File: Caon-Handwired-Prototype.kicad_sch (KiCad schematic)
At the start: 27 parts, among them SW1 SW_PUSH_MX, SW2 SW_PUSH_MX, SW3 SW_PUSH_MX, SW4 EC11 ENCODER 1, SW5 SW_PUSH_MX, SW6 SW_PUSH_MX, SW7 SW_PUSH_MX, SW8 EC11 ENCODER 1, U1 74HC595, U2 74HC595, U3 SuperMini nRF52840

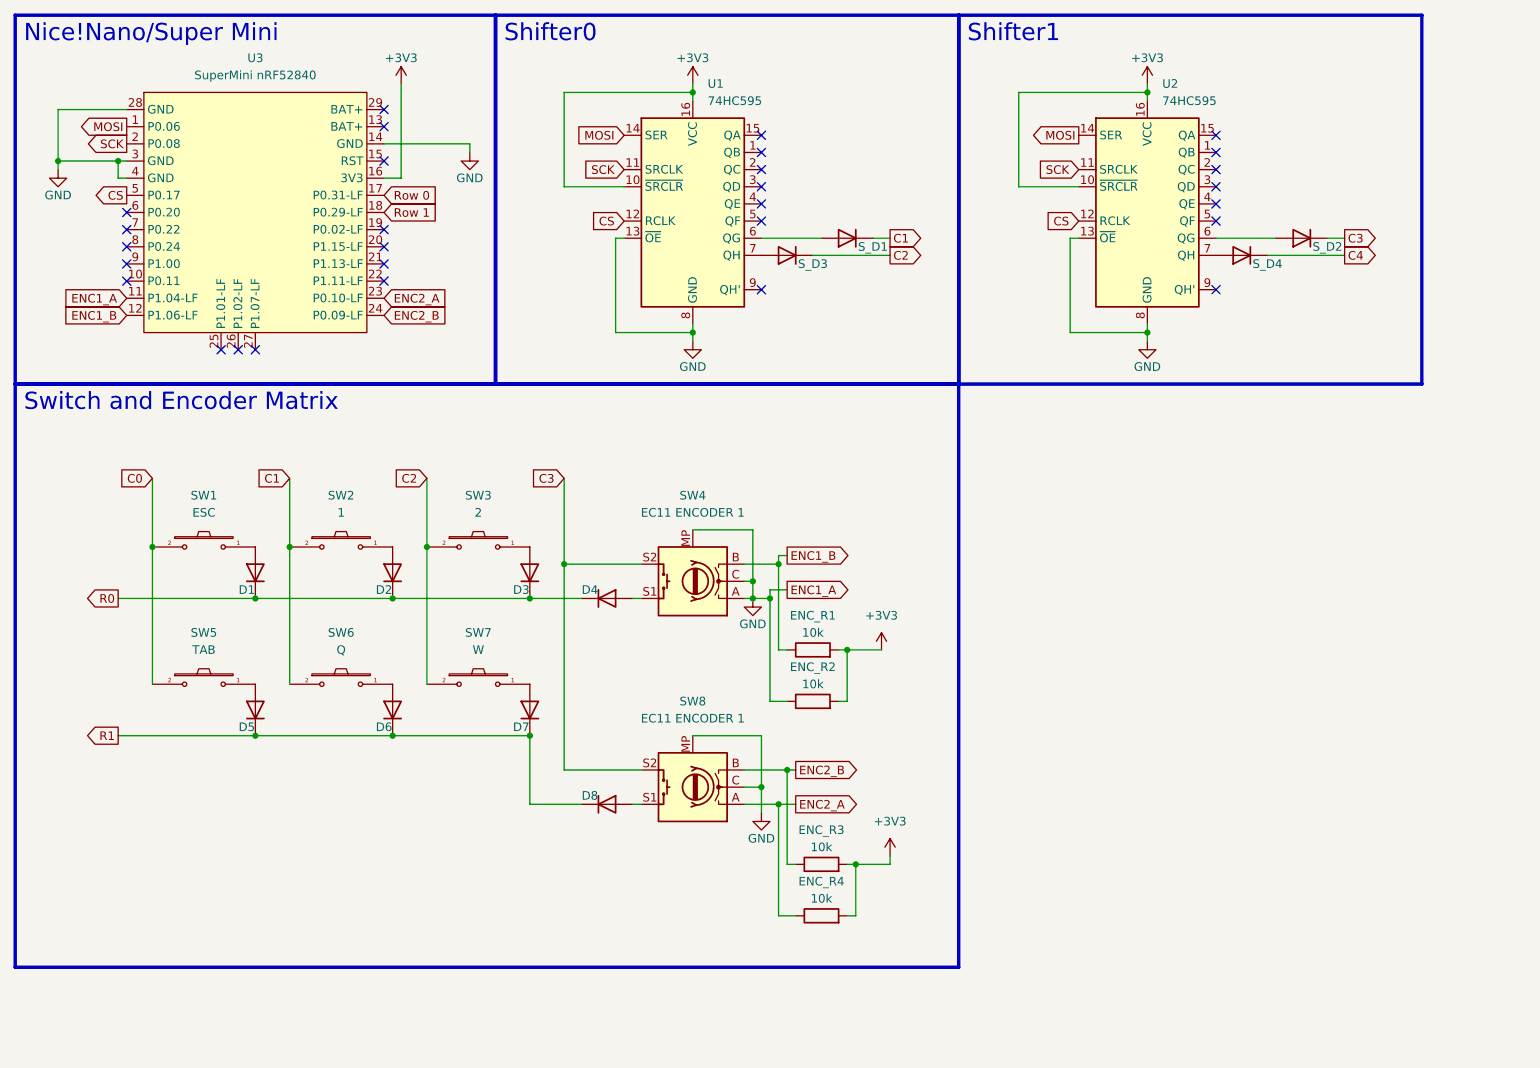
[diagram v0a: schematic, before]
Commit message: Update
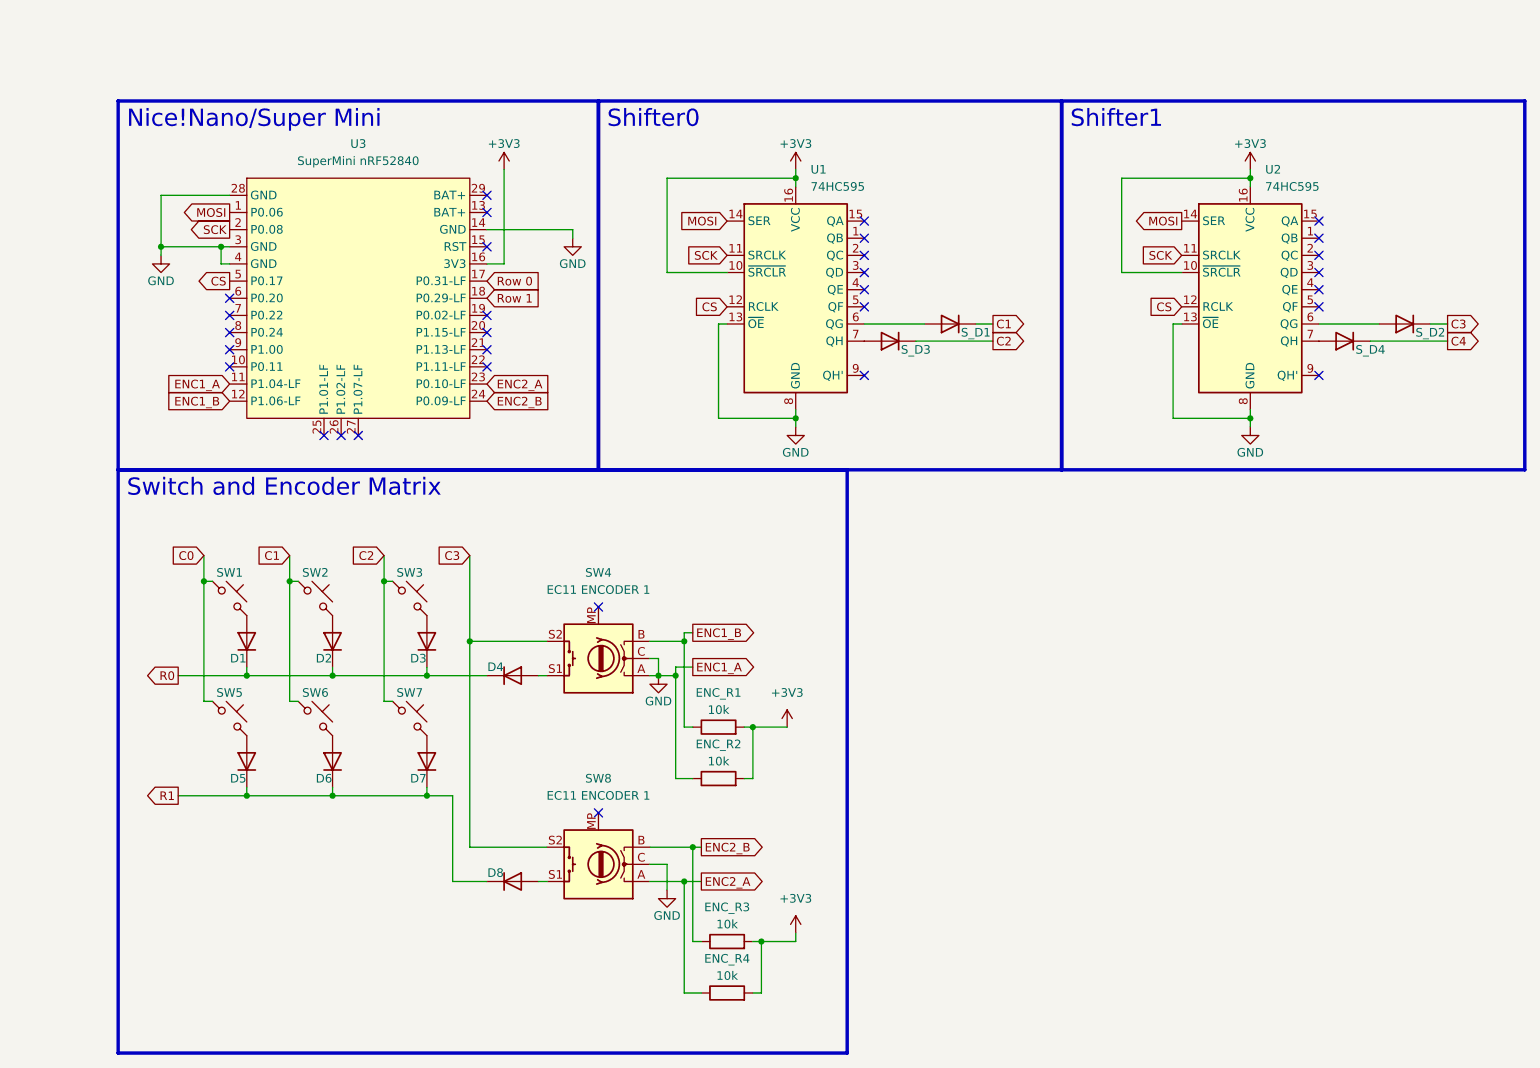
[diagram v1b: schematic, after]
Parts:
- removed SW1, SW2, SW3, SW5, SW6, SW7: SW_PUSH_MX, Caon_Footprint:SW_PUSH_6mm, symbol Caon65:SW_PUSH_MX
- added SW1, SW2, SW3, SW5, SW6, SW7: ~, Caon_Footprint:SW_PUSH_6mm, symbol Switch:SW_Push_45deg
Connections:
- net C0: now also SW1.1, SW5.1
- net C1: now also SW2.1, SW6.1
- net C2: now also SW3.1, SW7.1
- net GND: no longer SW4.MP, SW8.MP
- net at D1.2 (A): now also SW1.2
- net at D3.2 (A): now also SW3.2
- net at D5.2 (A): now also SW5.2
- net at D6.2 (A): now also SW6.2
- net at D2.2 (A): now also SW2.2
- net at D7.2 (A): now also SW7.2
- no-connect marks 29 -> 31
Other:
- moved on the sheet: D1, D4, D8, ENC_R1, ENC_R2, ENC_R3, ENC_R4, SW4, SW8, S_D1, S_D2, S_D3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

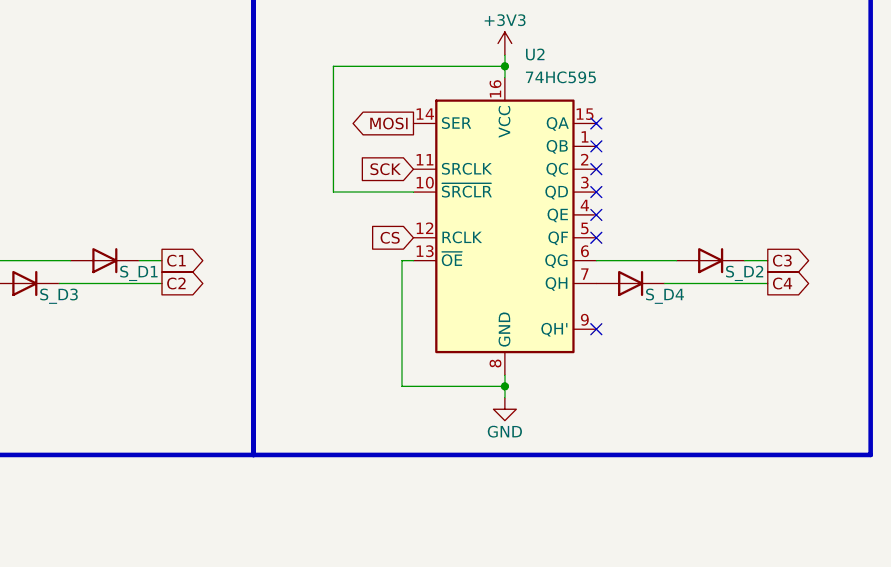
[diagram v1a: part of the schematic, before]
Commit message: Update
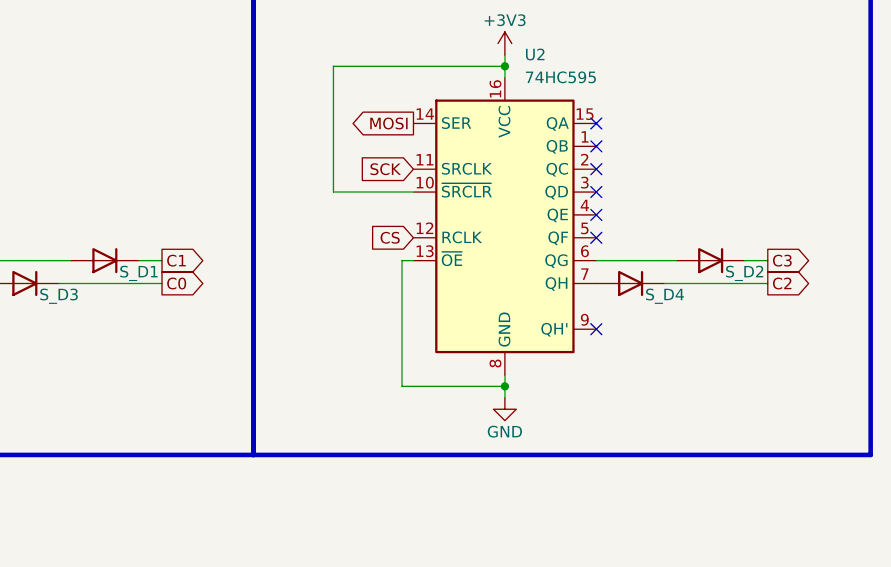
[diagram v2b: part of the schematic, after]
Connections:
- net C4 is gone; now on net C2: S_D4.1 (K)
- net C0: now also S_D3.1 (K)
- net C2: no longer S_D3.1 (K)

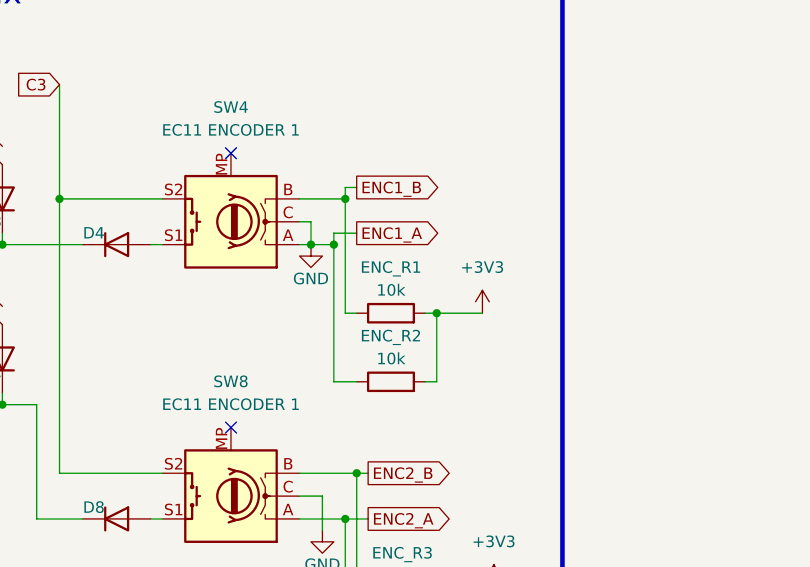
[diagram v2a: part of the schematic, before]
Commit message: Schematic Update
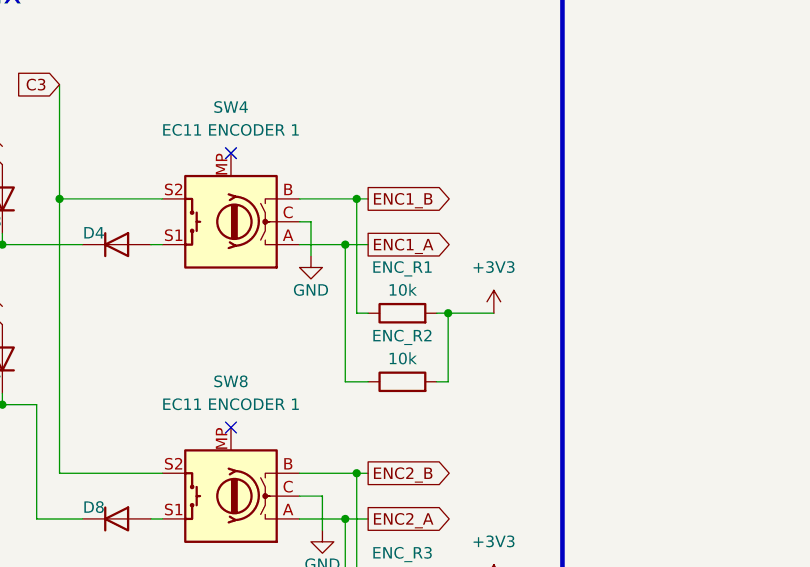
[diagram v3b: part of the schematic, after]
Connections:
- net GND: no longer ENC_R2.1, SW4.A, U3.11 (P1.04-LF)
- new net ENC1_A: ENC_R2.1, SW4.A, U3.11 (P1.04-LF)
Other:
- moved on the sheet: ENC_R1, ENC_R2
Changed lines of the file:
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@@
 	)
 	(junction
-		(at 137.16 125.73)
+		(at 138.43 125.73)
 		(diameter 0)
 		(color 0 0 0 0)
@@
 	)
 	(junction
-		(at 127 113.03)
+		(at 128.27 113.03)
 		(diameter 0)
 		(color 0 0 0 0)
@@
 	)
 	(junction
-		(at 123.19 118.11)
-		(diameter 0)
-		(color 0 0 0 0)
-	)
-	(junction
 		(at 138.43 157.48)
 		(diameter 0)
@@
 	)
 	(junction
-		(at 125.73 118.11)
+		(at 127 118.11)
 		(diameter 0)
 		(color 0 0 0 0)
@@
 	(wire
 		(pts
-			(xy 127 113.03) (xy 121.92 113.03)
-		)
-		(stroke
-			(width 0)
-			(type default)
-		)
-	)
-	(wire
-		(pts
-			(xy 127 125.73) (xy 127 113.03)
+			(xy 128.27 125.73) (xy 128.27 113.03)
 		)
 		(stroke
@@
 	(wire
 		(pts
-			(xy 127 113.03) (xy 127 111.76)
-		)
-		(stroke
-			(width 0)
-			(type default)
-		)
-	)
-	(wire
-		(pts
 			(xy 74.93 118.11) (xy 88.9 118.11)
 		)
@@
 	(wire
 		(pts
-			(xy 125.73 118.11) (xy 125.73 116.84)
-		)
-		(stroke
-			(width 0)
-			(type default)
-		)
-	)
-	(wire
-		(pts
 			(xy 137.16 165.1) (xy 138.43 165.1)
 		)
@@
 	(wire
 		(pts
-			(xy 127 111.76) (xy 128.27 111.76)
+			(xy 128.27 113.03) (xy 129.54 113.03)
 		)
 		(stroke
@@
 	(wire
 		(pts
-			(xy 123.19 118.11) (xy 123.19 115.57)
+			(xy 123.19 115.57) (xy 123.19 119.38)
 		)
 		(stroke
@@
 	(wire
 		(pts
-			(xy 128.27 125.73) (xy 127 125.73)
+			(xy 129.54 125.73) (xy 128.27 125.73)
 		)
 		(stroke
@@
 	(wire
 		(pts
-			(xy 125.73 133.35) (xy 125.73 118.11)
+			(xy 127 133.35) (xy 127 118.11)
 		)
 		(stroke
@@
 	(wire
 		(pts
-			(xy 137.16 133.35) (xy 137.16 125.73)
+			(xy 138.43 133.35) (xy 138.43 125.73)
 		)
 		(stroke
@@
 	(wire
 		(pts
-			(xy 135.89 125.73) (xy 137.16 125.73)
+			(xy 137.16 125.73) (xy 138.43 125.73)
 		)
 		(stroke
@@
 	(wire
 		(pts
-			(xy 125.73 118.11) (xy 123.19 118.11)
+			(xy 74.93 134.62) (xy 74.93 135.89)
 		)
 		(stroke
@@
 	(wire
 		(pts
-			(xy 74.93 134.62) (xy 74.93 135.89)
+			(xy 58.42 54.61) (xy 58.42 57.15)
 		)
 		(stroke
@@
 	(wire
 		(pts
-			(xy 58.42 54.61) (xy 58.42 57.15)
+			(xy 62.23 116.84) (xy 62.23 118.11)
 		)
 		(stroke
@@
 	(wire
 		(pts
-			(xy 62.23 116.84) (xy 62.23 118.11)
+			(xy 128.27 157.48) (xy 128.27 143.51)
 		)
 		(stroke
@@
 	(wire
 		(pts
-			(xy 128.27 157.48) (xy 128.27 143.51)
+			(xy 137.16 133.35) (xy 138.43 133.35)
 		)
 		(stroke
@@
 	(wire
 		(pts
-			(xy 135.89 133.35) (xy 137.16 133.35)
+			(xy 127 118.11) (xy 129.54 118.11)
 		)
 		(stroke
@@
 	(wire
 		(pts
-			(xy 125.73 116.84) (xy 128.27 116.84)
+			(xy 83.82 104.14) (xy 82.55 104.14)
 		)
 		(stroke
@@
 	(wire
 		(pts
-			(xy 83.82 104.14) (xy 82.55 104.14)
+			(xy 100.33 43.18) (xy 100.33 57.15)
 		)
 		(stroke
@@
 	(wire
 		(pts
-			(xy 100.33 43.18) (xy 100.33 57.15)
+			(xy 143.51 81.28) (xy 143.51 80.01)
 		)
 		(stroke
@@
 	(wire
 		(pts
-			(xy 143.51 81.28) (xy 143.51 80.01)
+			(xy 121.92 113.03) (xy 128.27 113.03)
 		)
 		(stroke
@@
 	(wire
 		(pts
-			(xy 128.27 133.35) (xy 125.73 133.35)
+			(xy 129.54 133.35) (xy 127 133.35)
 		)
 		(stroke
@@
 	(wire
 		(pts
-			(xy 123.19 118.11) (xy 121.92 118.11)
+			(xy 121.92 118.11) (xy 127 118.11)
 		)
 		(stroke
@@
 	(wire
 		(pts
-			(xy 137.16 125.73) (xy 142.24 125.73)
+			(xy 138.43 125.73) (xy 143.51 125.73)
 		)
 		(stroke
@@
 	(global_label "ENC1_A"
 		(shape output)
-		(at 128.27 116.84 0)
+		(at 129.54 118.11 0)
 		(fields_autoplaced yes)
 		(effects
@@
 		)
 		(property "Intersheetrefs" "${INTERSHEET_REFS}"
-			(at 138.2704 116.84 0)
+			(at 139.5404 118.11 0)
 			(effects
 				(font
@@
 	(global_label "ENC1_B"
 		(shape output)
-		(at 128.27 111.76 0)
+		(at 129.54 113.03 0)
 		(fields_autoplaced yes)
 		(effects
@@
 		)
 		(property "Intersheetrefs" "${INTERSHEET_REFS}"
-			(at 138.4518 111.76 0)
+			(at 139.7218 113.03 0)
 			(effects
 				(font
@@
 	(symbol
 		(lib_id "power:GND")
-		(at 123.19 118.11 0)
+		(at 123.19 119.38 0)
 		(unit 1)
 		(exclude_from_sim no)
@@
 		(dnp no)
 		(property "Reference" "#PWR08"
-			(at 123.19 124.46 0)
+			(at 123.19 125.73 0)
 			(effects
 				(font
@@
 		)
 		(property "Value" "GND"
-			(at 123.19 121.92 0)
+			(at 123.19 123.19 0)
 			(effects
 				(font
@@
 		)
 		(property "Footprint" ""
-			(at 123.19 118.11 0)
+			(at 123.19 119.38 0)
 			(effects
 				(font
@@
 		)
 		(property "Datasheet" ""
-			(at 123.19 118.11 0)
+			(at 123.19 119.38 0)
 			(effects
 				(font
@@
 		)
 		(property "Description" "Power symbol creates a global label with name \"GND\" , ground"
-			(at 123.19 118.11 0)
+			(at 123.19 119.38 0)
 			(effects
 				(font
@@
 	(symbol
 		(lib_id "Device:R")
-		(at 132.08 125.73 90)
+		(at 133.35 125.73 90)
 		(unit 1)
 		(exclude_from_sim no)
@@
 		(dnp no)
 		(property "Reference" "ENC_R1"
-			(at 132.08 120.65 90)
+			(at 133.35 120.65 90)
 			(effects
 				(font
@@
 		)
 		(property "Value" "10k"
-			(at 132.08 123.19 90)
+			(at 133.35 123.19 90)
 			(effects
 				(font
@@
 		)
 		(property "Footprint" "Resistor_THT:R_Axial_DIN0204_L3.6mm_D1.6mm_P2.54mm_Vertical"
-			(at 132.08 127.508 90)
+			(at 133.35 127.508 90)
 			(effects
 				(font
@@
 		)
 		(property "Datasheet" "~"
-			(at 132.08 125.73 0)
+			(at 133.35 125.73 0)
 			(effects
 				(font
@@
 		)
 		(property "Description" "Resistor"
-			(at 132.08 125.73 0)
+			(at 133.35 125.73 0)
 			(effects
 				(font
@@
 	(symbol
 		(lib_id "Device:R")
-		(at 132.08 133.35 90)
+		(at 133.35 133.35 90)
 		(unit 1)
 		(exclude_from_sim no)
@@
 		(dnp no)
 		(property "Reference" "ENC_R2"
-			(at 132.08 128.27 90)
+			(at 133.35 128.27 90)
 			(effects
 				(font
@@
 		)
 		(property "Value" "10k"
-			(at 132.08 130.81 90)
+			(at 133.35 130.81 90)
 			(effects
 				(font
@@
 		)
 		(property "Footprint" "Resistor_THT:R_Axial_DIN0204_L3.6mm_D1.6mm_P2.54mm_Vertical"
-			(at 132.08 135.128 90)
+			(at 133.35 135.128 90)
 			(effects
 				(font
@@
 		)
 		(property "Datasheet" "~"
-			(at 132.08 133.35 0)
+			(at 133.35 133.35 0)
 			(effects
 				(font
@@
 		)
 		(property "Description" "Resistor"
-			(at 132.08 133.35 0)
+			(at 133.35 133.35 0)
 			(effects
 				(font
@@
 	(symbol
 		(lib_id "power:VCC")
-		(at 142.24 125.73 0)
+		(at 143.51 125.73 0)
 		(unit 1)
 		(exclude_from_sim no)
@@
 		(dnp no)
 		(property "Reference" "#PWR09"
-			(at 142.24 129.54 0)
+			(at 143.51 129.54 0)
 			(effects
 				(font
@@
 		)
 		(property "Value" "+3V3"
-			(at 142.24 120.65 0)
+			(at 143.51 120.65 0)
 			(effects
 				(font
@@
 		)
 		(property "Footprint" ""
-			(at 142.24 125.73 0)
+			(at 143.51 125.73 0)
 			(effects
 				(font
@@
 		)
 		(property "Datasheet" ""
-			(at 142.24 125.73 0)
+			(at 143.51 125.73 0)
 			(effects
 				(font
@@
 		)
 		(property "Description" "Power symbol creates a global label with name \"VCC\""
-			(at 142.24 125.73 0)
+			(at 143.51 125.73 0)
 			(effects
 				(font

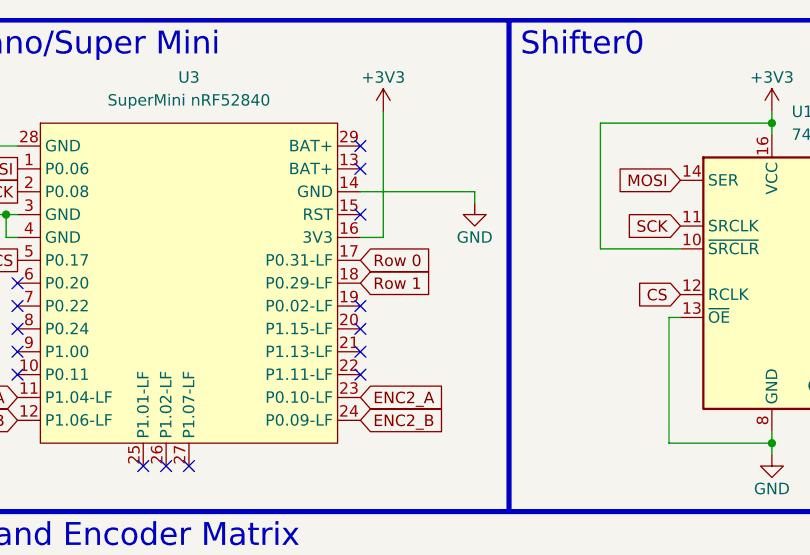
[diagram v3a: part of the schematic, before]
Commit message: Schematic update
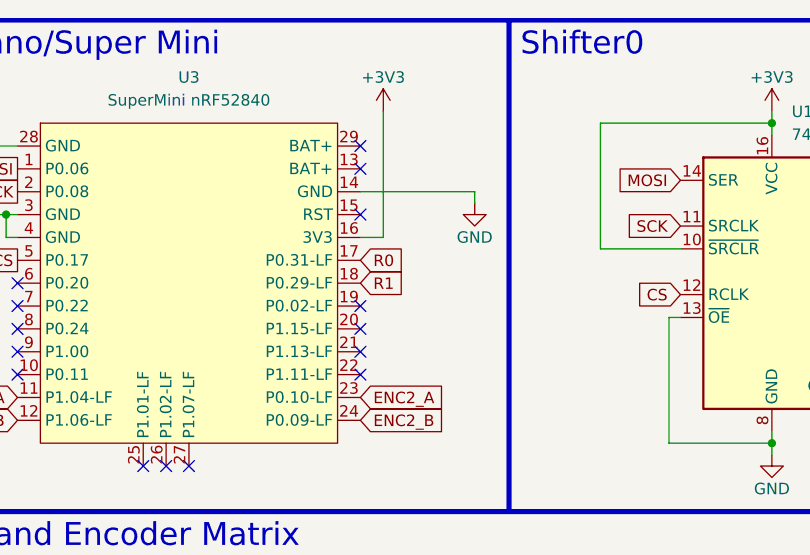
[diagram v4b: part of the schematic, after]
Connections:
- net Row 0 is gone; now on net R0: U3.17 (P0.31-LF)
- net Row 1 is gone; now on net R1: U3.18 (P0.29-LF)
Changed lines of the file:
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@@
 		)
 	)
-	(global_label "Row 0"
+	(global_label "R0"
 		(shape input)
 		(at 97.79 59.69 0)
@@
 		)
 		(property "Intersheetrefs" "${INTERSHEET_REFS}"
-			(at 106.7018 59.69 0)
+			(at 103.2547 59.69 0)
 			(effects
 				(font
@@
 		)
 	)
-	(global_label "Row 1"
+	(global_label "R1"
 		(shape input)
 		(at 97.79 62.23 0)
@@
 		)
 		(property "Intersheetrefs" "${INTERSHEET_REFS}"
-			(at 106.7018 62.23 0)
-			(effects
-				(font
+			(at 103.2547 62.23 0)
+			(effects
+				(font
